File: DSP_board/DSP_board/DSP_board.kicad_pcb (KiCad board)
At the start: 4 copper layers, 134.2 x 94.8 mm, 94 parts, among them IC1 SN74S1053NSR, IC5 F280025CPNQR, J1 Conn_01x02, J2 Conn_01x02, J3 Conn_01x02, J4 Conn_01x02, J5 1-84981-0, J6 Conn_01x02, J7 Conn_02x10_Odd_Even, J8 Conn_02x06_Odd_Even, J9 Conn_02x06_Odd_Even

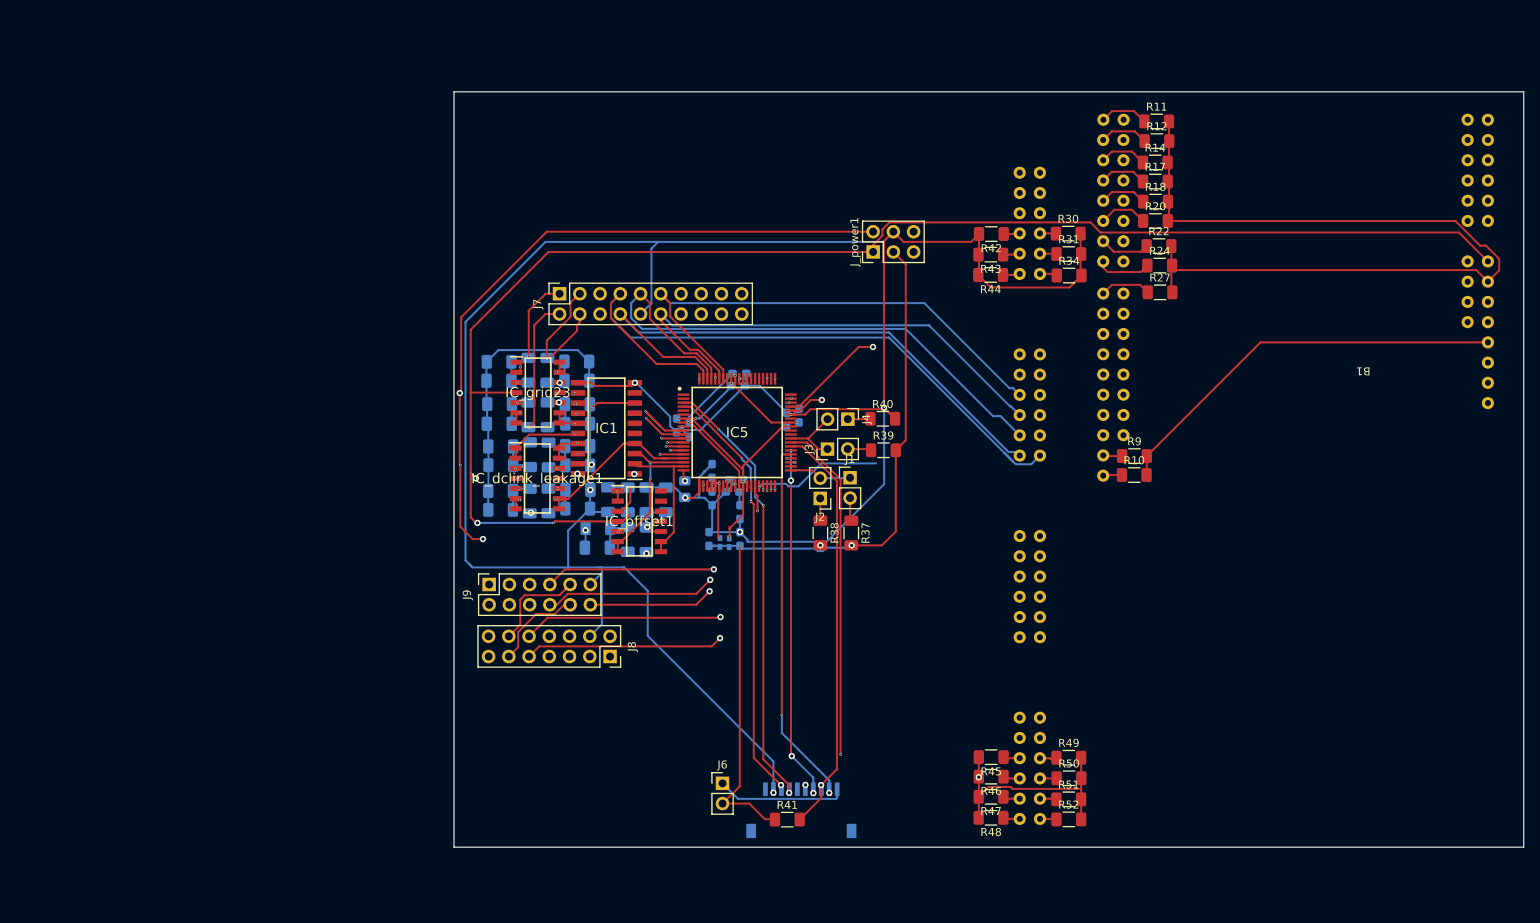
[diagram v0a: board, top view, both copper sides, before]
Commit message: header design
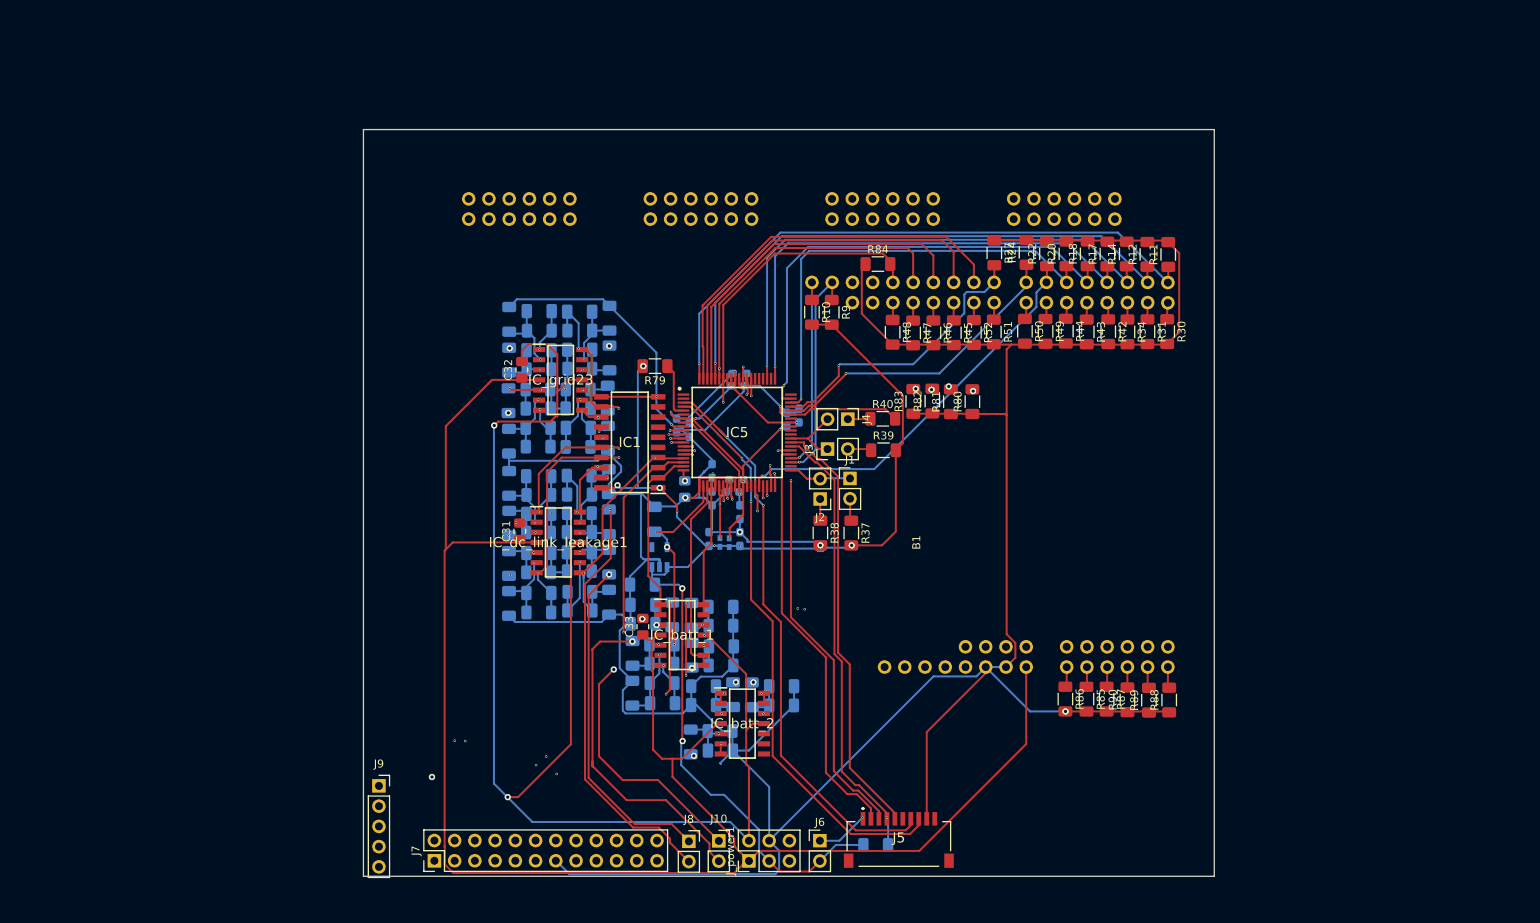
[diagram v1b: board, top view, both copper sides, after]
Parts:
- removed IC_dclink_leakage1, IC_offset1: LM324DR, lm324:SOIC127P600X175-14N
- added C12: CAP, Capacitor_SMD:C_1206_3216Metric_Pad1.33x1.80mm_HandSolder, B.Cu at (108.1, 74.1)
- added C13: CAP, Capacitor_SMD:C_1206_3216Metric_Pad1.33x1.80mm_HandSolder, B.Cu at (108.1, 109.5)
- added C20: CAP, Capacitor_SMD:C_1206_3216Metric_Pad1.33x1.80mm_HandSolder, B.Cu at (113.2, 111.7)
- added C21: CAP, Capacitor_SMD:C_1206_3216Metric_Pad1.33x1.80mm_HandSolder, B.Cu at (113.2, 74.2)
- added C22: CAP, Capacitor_SMD:C_1206_3216Metric_Pad1.33x1.80mm_HandSolder, B.Cu at (113.2, 97.2)
- added C23: CAP, Capacitor_SMD:C_1206_3216Metric_Pad1.33x1.80mm_HandSolder, B.Cu at (138.5, 121.2)
- added C24: CAP, Capacitor_SMD:C_1206_3216Metric_Pad1.33x1.80mm_HandSolder, B.Cu at (113.2, 104.4)
- added C25: CAP, Capacitor_SMD:C_1206_3216Metric_Pad1.33x1.80mm_HandSolder, B.Cu at (113.2, 101.9)
- added C26: CAP, Capacitor_SMD:C_1206_3216Metric_Pad1.33x1.80mm_HandSolder, B.Cu at (121.1, 111.0)
- added C27: CAP, Capacitor_SMD:C_1206_3216Metric_Pad1.33x1.80mm_HandSolder, B.Cu at (121.1, 108.5)
- added C28: CAP, Capacitor_SMD:C_1206_3216Metric_Pad1.33x1.80mm_HandSolder, B.Cu at (123.6, 123.3)
- added C29: CAP, Capacitor_SMD:C_1206_3216Metric_Pad1.33x1.80mm_HandSolder, B.Cu at (122.6, 100.3)
- added C30: CAP, Capacitor_SMD:C_1206_3216Metric_Pad1.33x1.80mm_HandSolder, B.Cu at (130.9, 111.2)
- added C31: CAP, Capacitor_SMD:C_0805_2012Metric_Pad1.18x1.45mm_HandSolder, F.Cu at (105.7, 101.8)
- added C32: CAP, Capacitor_SMD:C_0805_2012Metric_Pad1.18x1.45mm_HandSolder, F.Cu at (105.9, 81.5)
- added C33: CAP, Capacitor_SMD:C_0805_2012Metric_Pad1.18x1.45mm_HandSolder, F.Cu at (121.1, 113.7)
- added C5: CAP, Capacitor_SMD:C_1206_3216Metric_Pad1.33x1.80mm_HandSolder, B.Cu at (108.1, 104.5)
- added C6: CAP, Capacitor_SMD:C_1206_3216Metric_Pad1.33x1.80mm_HandSolder, B.Cu at (108.1, 99.6)
- added C8: CAP, Capacitor_SMD:C_1206_3216Metric_Pad1.33x1.80mm_HandSolder, B.Cu at (128.8, 123.6)
- added IC_batt_1: LM324DR, lm324:SOIC127P600X175-14N, F.Cu at (126.0, 114.8)
- added IC_batt_2: LM324DR, lm324:SOIC127P600X175-14N, F.Cu at (133.6, 125.9)
- added IC_dc_link_leakage1: LM324DR, lm324:SOIC127P600X175-14N, F.Cu at (110.5, 103.2)
- added J10: Conn_02x01, Connector_PinSocket_2.54mm:PinSocket_1x02_P2.54mm_Vertical, F.Cu at (130.7, 140.6)
- added LDO1: NCV8114ASN165T1G, ldo_ncv118:SOT95P275X110-5N, B.Cu at (123.2, 105.0)
- added R53: R, Resistor_SMD:R_1206_3216Metric_Pad1.30x1.75mm_HandSolder, B.Cu at (108.0, 91.1)
- added R54: R, Resistor_SMD:R_1206_3216Metric_Pad1.30x1.75mm_HandSolder, B.Cu at (108.1, 97.2)
- added R55: R, Resistor_SMD:R_1206_3216Metric_Pad1.30x1.75mm_HandSolder, B.Cu at (108.1, 111.9)
- added R56: R, Resistor_SMD:R_1206_3216Metric_Pad1.30x1.75mm_HandSolder, B.Cu at (132.4, 122.3)
- added R57: R, Resistor_SMD:R_1206_3216Metric_Pad1.30x1.75mm_HandSolder, B.Cu at (127.1, 128.2)
- added R58: R, Resistor_SMD:R_1206_3216Metric_Pad1.30x1.75mm_HandSolder, B.Cu at (134.8, 122.3)
- added R59: R, Resistor_SMD:R_1206_3216Metric_Pad1.30x1.75mm_HandSolder, B.Cu at (116.7, 90.1)
- added R60: R, Resistor_SMD:R_1206_3216Metric_Pad1.30x1.75mm_HandSolder, B.Cu at (113.2, 76.6)
- added R61: R, Resistor_SMD:R_1206_3216Metric_Pad1.30x1.75mm_HandSolder, B.Cu at (116.9, 110.7)
- added R62: R, Resistor_SMD:R_1206_3216Metric_Pad1.30x1.75mm_HandSolder, B.Cu at (113.0, 91.2)
- added R63: R, Resistor_SMD:R_1206_3216Metric_Pad1.30x1.75mm_HandSolder, B.Cu at (113.1, 94.8)
- added R64: R, Resistor_SMD:R_1206_3216Metric_Pad1.30x1.75mm_HandSolder, B.Cu at (113.2, 109.4)
- added R65: R, Resistor_SMD:R_1206_3216Metric_Pad1.30x1.75mm_HandSolder, B.Cu at (138.5, 123.6)
- added R66: R, Resistor_SMD:R_1206_3216Metric_Pad1.30x1.75mm_HandSolder, B.Cu at (116.9, 105.6)
- added R67: R, Resistor_SMD:R_1206_3216Metric_Pad1.30x1.75mm_HandSolder, B.Cu at (117.0, 75.0)
- added R68: R, Resistor_SMD:R_1206_3216Metric_Pad1.30x1.75mm_HandSolder, B.Cu at (113.0, 84.0)
- added R69: R, Resistor_SMD:R_1206_3216Metric_Pad1.30x1.75mm_HandSolder, B.Cu at (116.8, 95.5)
- added R70: R, Resistor_SMD:R_1206_3216Metric_Pad1.30x1.75mm_HandSolder, B.Cu at (113.2, 106.8)
- added R71: R, Resistor_SMD:R_1206_3216Metric_Pad1.30x1.75mm_HandSolder, B.Cu at (116.9, 100.6)
- added R72: R, Resistor_SMD:R_1206_3216Metric_Pad1.30x1.75mm_HandSolder, B.Cu at (113.2, 99.5)
- added R73: R, Resistor_SMD:R_1206_3216Metric_Pad1.30x1.75mm_HandSolder, B.Cu at (121.2, 113.4)
- added R74: R, Resistor_SMD:R_1206_3216Metric_Pad1.30x1.75mm_HandSolder, B.Cu at (123.5, 120.8)
- added R75: R, Resistor_SMD:R_1206_3216Metric_Pad1.30x1.75mm_HandSolder, B.Cu at (124.8, 112.3)
- added R76: R, Resistor_SMD:R_1206_3216Metric_Pad1.30x1.75mm_HandSolder, B.Cu at (130.9, 113.6)
- added R77: R, Resistor_SMD:R_1206_3216Metric_Pad1.30x1.75mm_HandSolder, B.Cu at (127.2, 112.3)
- added R78: R, Resistor_SMD:R_1206_3216Metric_Pad1.30x1.75mm_HandSolder, B.Cu at (119.8, 122.1)
- added R79: R, Resistor_SMD:R_1206_3216Metric_Pad1.30x1.75mm_HandSolder, F.Cu at (122.7, 81.0)
- added R80: R, Resistor_SMD:R_1206_3216Metric_Pad1.30x1.75mm_HandSolder, F.Cu at (162.5, 85.5)
- added R81: R, Resistor_SMD:R_1206_3216Metric_Pad1.30x1.75mm_HandSolder, F.Cu at (159.8, 85.5)
- added R82: R, Resistor_SMD:R_1206_3216Metric_Pad1.30x1.75mm_HandSolder, F.Cu at (157.5, 85.4)
- added R83: R, Resistor_SMD:R_1206_3216Metric_Pad1.30x1.75mm_HandSolder, F.Cu at (155.1, 85.5)
- added R84: R, Resistor_SMD:R_1206_3216Metric_Pad1.30x1.75mm_HandSolder, F.Cu at (150.6, 68.2)
- added R85: R, Resistor_SMD:R_1206_3216Metric_Pad1.30x1.75mm_HandSolder, F.Cu at (176.8, 122.8)
- added R86: R, Resistor_SMD:R_1206_3216Metric_Pad1.30x1.75mm_HandSolder, F.Cu at (174.2, 122.8)
- added R87: R, Resistor_SMD:R_1206_3216Metric_Pad1.30x1.75mm_HandSolder, F.Cu at (179.3, 122.8)
- added R88: R, Resistor_SMD:R_1206_3216Metric_Pad1.30x1.75mm_HandSolder, F.Cu at (187.2, 122.9)
- added R89: R, Resistor_SMD:R_1206_3216Metric_Pad1.30x1.75mm_HandSolder, F.Cu at (184.7, 123.0)
- added R90: R, Resistor_SMD:R_1206_3216Metric_Pad1.30x1.75mm_HandSolder, F.Cu at (181.9, 122.9)
- J5: moved to F.Cu
- J7: value Conn_02x10_Odd_Even -> Conn_02x12_Odd_Even; footprint Connector_PinSocket_2.54mm:PinSocket_2x10_P2.54mm_Vertical -> Connector_PinHeader_2.54mm:PinHeader_2x12_P2.54mm_Vertical
- J8: value Conn_02x06_Odd_Even -> Conn_02x01; footprint Connector_PinSocket_2.54mm:PinSocket_2x07_P2.54mm_Vertical -> Connector_PinSocket_2.54mm:PinSocket_1x02_P2.54mm_Vertical
- J9: value Conn_02x06_Odd_Even -> Conn_01x05; footprint Connector_PinSocket_2.54mm:PinSocket_2x06_P2.54mm_Vertical -> Connector_PinSocket_2.54mm:PinSocket_1x05_P2.54mm_Vertical
- R41: moved to B.Cu
- moved J_power1 78.0 mm to (134.4, 143.1)
- moved J7 72.9 mm to (95.0, 143.1)
- moved B1 67.0 mm to (155.0, 108.3), turned to 90 degrees
- moved R52 62.3 mm to (162.7, 76.8), turned to -90 degrees
- moved R48 62.2 mm to (152.5, 76.8), turned to -90 degrees
- moved R51 59.4 mm to (165.2, 76.7), turned to -90 degrees
- moved R47 59.0 mm to (155.1, 76.9), turned to -90 degrees
- moved R50 56.4 mm to (169.1, 76.7), turned to -90 degrees
- moved R46 56.2 mm to (157.6, 76.8), turned to -90 degrees
- moved R49 53.6 mm to (171.7, 76.7), turned to -90 degrees
- moved R45 53.5 mm to (160.2, 76.8), turned to -90 degrees
- moved C10 47.1 mm to (130.9, 129.3), turned to 0 degrees
- moved R10 45.3 mm to (142.3, 74.3), turned to -90 degrees
- moved R9 42.1 mm to (144.8, 74.3), turned to -90 degrees
- moved R33 36.0 mm to (130.8, 126.8), turned to 180 degrees
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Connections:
- B1 pad 102: VSI11 -> unconnected-(B1-Pad102)
- B1 pad 103: VSI21 -> unconnected-(B1-Pad103)
- B1 pad 104: VSI31 -> unconnected-(B1-Pad104)
- B1 pad 14: unconnected-(B1-Pad14) -> OCD_grid1
- B1 pad 15: unconnected-(B1-Pad15) -> OCD_grd2
- B1 pad 16: unconnected-(B1-Pad16) -> OCD_grid3
- B1 pad 17: unconnected-(B1-Pad17) -> relay_3
- B1 pad 18: unconnected-(B1-Pad18) -> relay_2
- B1 pad 19: unconnected-(B1-Pad19) -> relay_1
- B1 pad 26: unconnected-(B1-Pad26) -> batt_ready
- B1 pad 27: unconnected-(B1-Pad27) -> batt_fault
- B1 pad 28: unconnected-(B1-Pad28) -> DAB2_PWM22
- B1 pad 29: unconnected-(B1-Pad29) -> DAB2_PWM21
- B1 pad 30: unconnected-(B1-Pad30) -> DAB2_PWM12
- B1 pad 31: unconnected-(B1-Pad31) -> DAB2_PWM11
- B1 pad 32: unconnected-(B1-Pad32) -> DAB1PWM22
- B1 pad 33: unconnected-(B1-Pad33) -> DAB1PWM21
- B1 pad 34: unconnected-(B1-Pad34) -> DAB1PWM12
- B1 pad 35: unconnected-(B1-Pad35) -> DAB1PWM11
- B1 pad 36: unconnected-(B1-Pad36) -> VSI32
- B1 pad 37: unconnected-(B1-Pad37) -> VSI31
- B1 pad 38: unconnected-(B1-Pad38) -> VSI22
- B1 pad 39: unconnected-(B1-Pad39) -> VSI21
- B1 pad 40: unconnected-(B1-Pad40) -> VSI12
- B1 pad 41: unconnected-(B1-Pad41) -> VSI11
- B1 pad 46: unconnected-(B1-Pad46) -> vsi_ready
- B1 pad 47: unconnected-(B1-Pad47) -> vsi_fault
- B1 pad 48: unconnected-(B1-Pad48) -> OCD_leakage
- B1 pad 49: unconnected-(B1-Pad49) -> dc_fault
- B1 pad 50: unconnected-(B1-Pad50) -> dc_ready
- B1 pad 60: DAB1PWM22 -> unconnected-(B1-Pad60)
- B1 pad 61: DAB1PWM21 -> unconnected-(B1-Pad61)
- B1 pad 62: DAB1PWM12 -> unconnected-(B1-Pad62)
- B1 pad 63: DAB1PWM11 -> unconnected-(B1-Pad63)
- B1 pad 66: DAB2_PWM22 -> unconnected-(B1-Pad66)
- B1 pad 67: DAB2_PWM21 -> unconnected-(B1-Pad67)
- B1 pad 68: DAB2_PWM12 -> unconnected-(B1-Pad68)
- B1 pad 69: DAB2_PWM11 -> unconnected-(B1-Pad69)
- B1 pad 84: OCD_grid1 -> unconnected-(B1-Pad84)
- B1 pad 90: OCD_grd2 -> unconnected-(B1-Pad90)
- B1 pad 91: OCD_grid3 -> unconnected-(B1-Pad91)
- B1 pad 92: vsi_fault -> unconnected-(B1-Pad92)
- B1 pad 93: vsi_ready -> unconnected-(B1-Pad93)
- B1 pad 96: VSI12 -> unconnected-(B1-Pad96)
- B1 pad 97: VSI22 -> unconnected-(B1-Pad97)
- B1 pad 98: VSI32 -> unconnected-(B1-Pad98)
- C10 pad 2: offset_v -> ctrl_gnd
- C11 pad 1: Net-(C11-Pad1) -> Vgrid3_sense
- C11 pad 2: offset_v -> Net-(C11-Pad2)
- C14 pad 1: Net-(C14-Pad1) -> Igrid1_sense
- C14 pad 2: ctrl_gnd -> Net-(C14-Pad2)
- C15 pad 2: offset_v -> Vgrid2_sense
- IC1 pad 13: Igrid3_sense -> Vgrid2_sense
- IC1 pad 14: Vgrid3_sense -> Igrid3_sense
- IC1 pad 15: Vgrid2_sense -> Vgrid3_sense
- IC1 pad 17: I_leackage -> Vgrid1_sense
- IC1 pad 18: Vgrid1_sense -> I_leackage
- IC1 pad 19: unconnected-(IC1-Pad19) -> offset_v
- IC1 pad 8: offset_v -> unconnected-(IC1-Pad8)
- IC5 pad 11: Igrid3_sense -> Vgrid2_sense
- IC5 pad 12: Vgrid3_sense -> Igrid3_sense
- IC5 pad 13: Vgrid2_sense -> Vgrid3_sense
- IC5 pad 15: I_leackage -> Vgrid1_sense
- IC5 pad 16: Vgrid1_sense -> I_leackage
- IC5 pad 23: unconnected-(IC5-Pad23) -> ADC1
- IC5 pad 24: unconnected-(IC5-Pad24) -> ADC2
- IC5 pad 27: unconnected-(IC5-Pad27) -> ADC3
- IC5 pad 28: unconnected-(IC5-Pad28) -> ADC4
- IC5 pad 29: unconnected-(IC5-Pad29) -> ADC5
- IC5 pad 35: dc_ready -> OCD_grid1
- IC5 pad 37: dc_fault -> OCD_grd2
- IC5 pad 38: OCD_leakage -> OCD_grid3
- IC5 pad 5: unconnected-(IC5-Pad5) -> Net-(IC5-Pad5)
- IC5 pad 56: /controller_sheet/en_dab -> /controller_sheet/en_vsi
- IC5 pad 57: /controller_sheet/en_vsi -> /controller_sheet/en_dab
- IC5 pad 67: unconnected-(IC5-Pad67) -> relay_3
- IC5 pad 68: unconnected-(IC5-Pad68) -> relay_2
- IC5 pad 69: unconnected-(IC5-Pad69) -> relay_1
- IC5 pad 77: OCD_grid3 -> OCD_leakage
- IC5 pad 78: OCD_grd2 -> dc_fault
- IC5 pad 79: OCD_grid1 -> dc_ready
- IC_grid23 pad 13: Igrid2_sense -> Net-(C21-Pad2)
- IC_grid23 pad 2: Igrid3_sense -> Net-(C12-Pad2)
- IC_grid23 pad 6: Vgrid3_sense -> Net-(C11-Pad2)
- IC_grid23 pad 9: Vgrid2_sense -> Net-(C15-Pad1)
- J5 pad 3: TMS -> TDO
- J5 pad 4: TDO -> TMS
- J7 pad 1: Igrid3 -> relay_3
- J7 pad 10: ctrl_gnd -> Igrid1
- J7 pad 11: vsi_ready -> OCD_grd2
- J7 pad 12: vsi_fault -> OCD_grid1
- J7 pad 13: VSI31 -> ctrl_gnd
- J7 pad 14: VSI32 -> OCD_grid3
- J7 pad 15: VSI21 -> vsi_fault
- J7 pad 16: VSI22 -> vsi_ready
- J7 pad 17: VSI11 -> VSI31
- J7 pad 18: VSI12 -> VSI32
- J7 pad 19: SCL -> VSI21
- J7 pad 2: Vgrid3 -> unconnected-(J7-Pad2)
- J7 pad 20: SDA -> VSI22
- J7 pad 3: Igrid2 -> relay_2
- J7 pad 4: Vgrid2 -> relay_1
- J7 pad 5: Igrid1 -> Vgrid3
- J7 pad 6: Vgrid1 -> Igrid3
- J7 pad 7: OCD_grid1 -> Vgrid2
- J7 pad 8: OCD_grd2 -> Igrid2
- J7 pad 9: OCD_grid3 -> Vgrid1
- J8 pad 1: batt_curr_0 -> V_dc_link
- J8 pad 2: batt_v -> curr_leakeage_i
- J9 pad 1: curr_leakeage_i -> Analog_in1
- J9 pad 2: V_dc_link -> Analog_in2
- J9 pad 3: DAB1PWM21 -> Analog_in3
- J9 pad 4: DAB1PWM22 -> Analog_in4
- J9 pad 5: DAB1PWM11 -> Analog_in5
- R10 pad 2: FPGA_3v3 -> ctrl_3v3
- R13 pad 1: Net-(IC_offset1-Pad3) -> offset_v
- R13 pad 2: ctrl_15 -> Net-(C5-Pad1)
- R15 pad 1: Net-(IC_offset1-Pad3) -> offset_v
- R15 pad 2: ctrl_gnd -> Net-(C6-Pad1)
- R19 pad 1: offset_v -> Net-(C6-Pad1)
- R19 pad 2: Net-(C7-Pad1) -> Igrid1
- R25 pad 1: offset_v -> Vgrid1
- R25 pad 2: Net-(C10-Pad1) -> Net-(C5-Pad1)
- R26 pad 1: Net-(C10-Pad1) -> ctrl_gnd
- R26 pad 2: Igrid1 -> Net-(C12-Pad2)
- R27 pad 1: /controller_sheet/en_dab -> ctrl_gnd
- R27 pad 2: ctrl_gnd -> /controller_sheet/en_dab
- R28 pad 1: offset_v -> ctrl_gnd
- R28 pad 2: Net-(C11-Pad1) -> Net-(C14-Pad2)
- R29 pad 1: Vgrid1 -> ctrl_gnd
- R29 pad 2: Net-(C11-Pad1) -> Net-(C11-Pad2)
- R30 pad 1: VSI32 -> VSI11
- R31 pad 1: VSI22 -> VSI12
- R32 pad 2: Net-(C14-Pad1) -> Net-(C8-Pad1)
- R33 pad 1: V_dc_link -> ctrl_gnd
- R33 pad 2: Net-(C14-Pad1) -> Net-(C10-Pad1)
- R34 pad 1: VSI12 -> VSI21
- R35 pad 1: Net-(C15-Pad1) -> ctrl_gnd
- R35 pad 2: curr_leakeage_i -> Net-(C13-Pad2)
- R36 pad 1: offset_v -> Net-(C12-Pad2)
- R36 pad 2: Net-(C15-Pad1) -> Igrid3_sense
- R42 pad 1: VSI31 -> VSI22
- R43 pad 1: VSI21 -> VSI31
- R44 pad 1: VSI11 -> VSI32
- R9 pad 2: FPGA_3v3 -> ctrl_3v3
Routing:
- net relay_1: track 0.00 -> 149.2 mm, vias 0 -> 2
- net relay_3: track 0.00 -> 146.3 mm, vias 0 -> 2
- net relay_2: track 0.00 -> 144.4 mm, vias 0 -> 2
- net DAB1PWM22: track 87.3 -> 2.20 mm
- net DAB1PWM21: track 86.7 -> 2.14 mm
- net DAB1PWM11: track 79.5 -> 2.11 mm
- net DAB1PWM12: track 78.5 -> 2.12 mm
- net ctrl_gnd: track 609.5 -> 534.1 mm, vias 12 -> 9
- net DAB2_PWM22: track 70.4 -> 2.18 mm
- net DAB2_PWM11: track 68.7 -> 2.24 mm
- net DAB2_PWM21: track 68.6 -> 2.25 mm
- net VSI11: track 40.6 -> 104.5 mm
- net DAB2_PWM12: track 66.0 -> 2.24 mm
- net vsi_fault: track 62.1 -> 125.3 mm, vias 0 -> 2
- net Igrid2: track 9.86 -> 70.6 mm
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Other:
- board size 134.2 x 94.8 mm -> 106.8 x 93.7 mm

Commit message: review changes
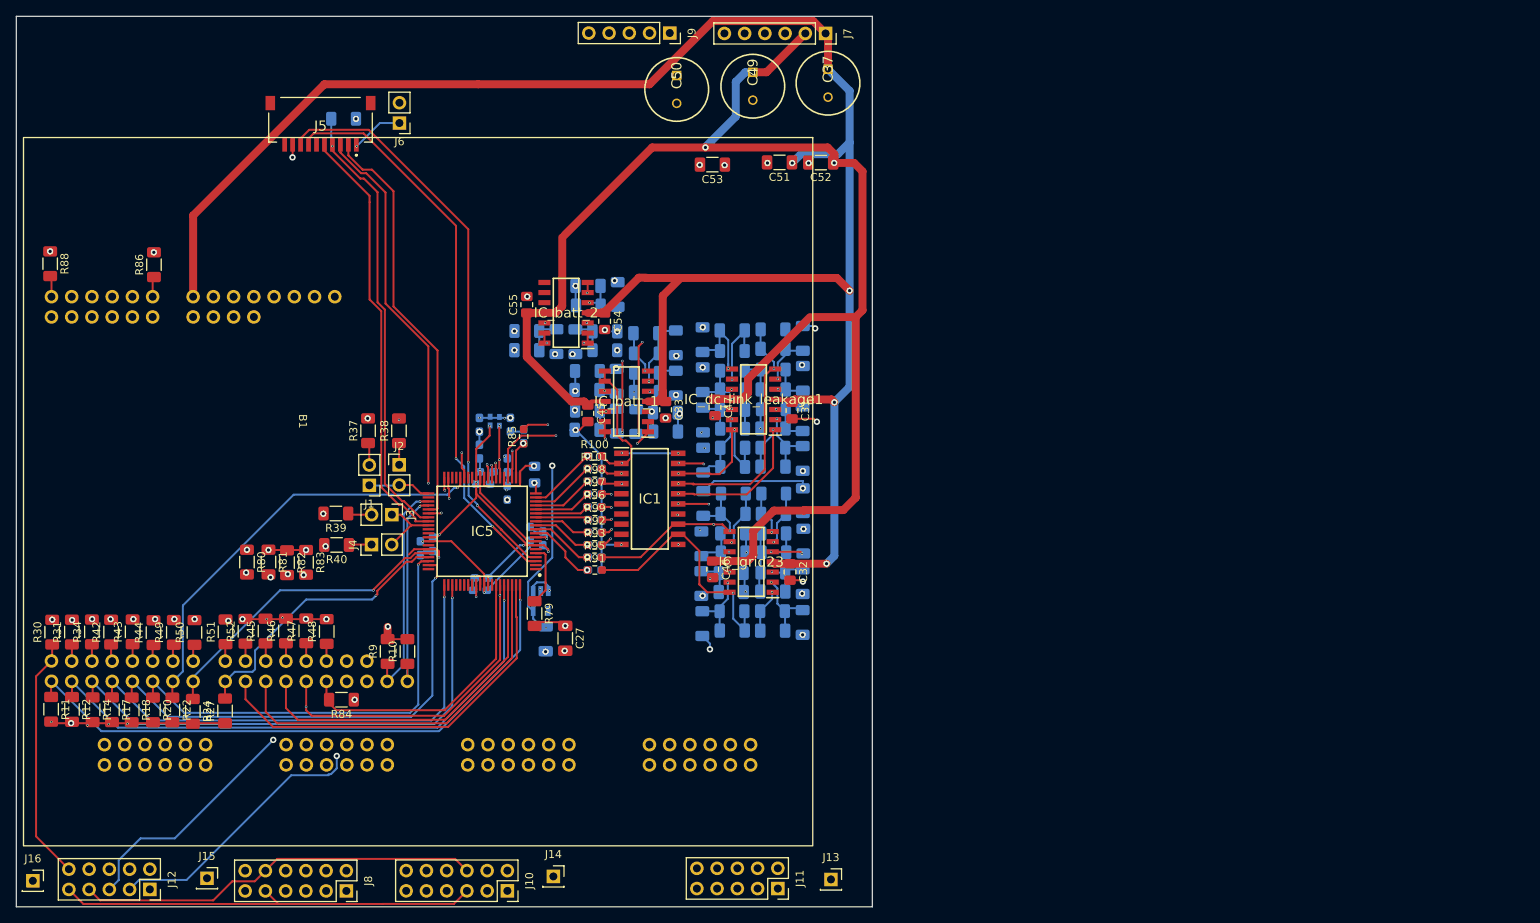
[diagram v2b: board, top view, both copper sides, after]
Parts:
- removed J_power1: Conn_02x03_Counter_Clockwise, Connector_PinHeader_2.54mm:PinHeader_2x03_P2.54mm_Vertical
- removed R87, R89, R90: R, Resistor_SMD:R_1206_3216Metric_Pad1.30x1.75mm_HandSolder
- added C34: CAP, Capacitor_SMD:C_0603_1608Metric_Pad1.08x0.95mm_HandSolder, B.Cu at (115.1, 106.6)
- added C35: CAP, Capacitor_SMD:C_0603_1608Metric_Pad1.08x0.95mm_HandSolder, B.Cu at (115.1, 101.9)
- added C36: CAP, Capacitor_SMD:C_0603_1608Metric_Pad1.08x0.95mm_HandSolder, B.Cu at (115.1, 103.4)
- added C37: ESK107M050AG3EA, electrolytic_cap:CAPPRD350W60D800H1250, F.Cu at (144.4, 43.8)
- added C38: CAP, Capacitor_SMD:C_0603_1608Metric_Pad1.08x0.95mm_HandSolder, B.Cu at (115.1, 105.0)
- added C39: CAP, Capacitor_SMD:C_0603_1608Metric_Pad1.08x0.95mm_HandSolder, B.Cu at (115.0, 98.7)
- added C40: CAP, Capacitor_SMD:C_0603_1608Metric_Pad1.08x0.95mm_HandSolder, B.Cu at (115.1, 97.1)
- added C41: CAP, Capacitor_SMD:C_0603_1608Metric_Pad1.08x0.95mm_HandSolder, B.Cu at (115.1, 95.5)
- added C42: CAP, Capacitor_SMD:C_0603_1608Metric_Pad1.08x0.95mm_HandSolder, B.Cu at (115.1, 100.3)
- added C43: CAP, Capacitor_SMD:C_0603_1608Metric_Pad1.08x0.95mm_HandSolder, B.Cu at (115.1, 92.3)
- added C44: CAP, Capacitor_SMD:C_0603_1608Metric_Pad1.08x0.95mm_HandSolder, B.Cu at (115.1, 93.9)
- added C45: CAP, Capacitor_SMD:C_0805_2012Metric_Pad1.18x1.45mm_HandSolder, F.Cu at (114.2, 87.0)
- added C46: CAP, Capacitor_SMD:C_0805_2012Metric_Pad1.18x1.45mm_HandSolder, F.Cu at (129.9, 106.5)
- added C47: CAP, Capacitor_SMD:C_0805_2012Metric_Pad1.18x1.45mm_HandSolder, F.Cu at (130.2, 86.2)
- added C48: CAP, Capacitor_SMD:C_0603_1608Metric_Pad1.08x0.95mm_HandSolder, B.Cu at (106.2, 89.8)
- added C49: ESK107M050AG3EA, electrolytic_cap:CAPPRD350W60D800H1250, F.Cu at (134.9, 44.1)
- added C50: ESK107M050AG3EA, electrolytic_cap:CAPPRD350W60D800H1250, F.Cu at (125.4, 44.5)
- added C51: CAP, Capacitor_SMD:C_1206_3216Metric_Pad1.33x1.80mm_HandSolder, F.Cu at (138.3, 55.5)
- added C52: CAP, Capacitor_SMD:C_1206_3216Metric_Pad1.33x1.80mm_HandSolder, F.Cu at (143.5, 55.5)
- added C53: CAP, Capacitor_SMD:C_1206_3216Metric_Pad1.33x1.80mm_HandSolder, F.Cu at (129.9, 55.7)
- added C54: CAP, Capacitor_SMD:C_0805_2012Metric_Pad1.18x1.45mm_HandSolder, F.Cu at (116.3, 75.4)
- added C55: CAP, Capacitor_SMD:C_0805_2012Metric_Pad1.18x1.45mm_HandSolder, F.Cu at (106.6, 73.3)
- added J11: Conn_02x05_Odd_Even, Connector_PinSocket_2.54mm:PinSocket_2x05_P2.54mm_Vertical, F.Cu at (138.1, 146.6)
- added J12: Conn_02x05_Odd_Even, Connector_PinSocket_2.54mm:PinSocket_2x05_P2.54mm_Vertical, F.Cu at (59.2, 146.7)
- added J13: Conn_01x01_Female, Connector_PinSocket_2.54mm:PinSocket_1x01_P2.54mm_Vertical, F.Cu at (144.7, 145.5)
- added J14: Conn_01x01_Female, Connector_PinSocket_2.54mm:PinSocket_1x01_P2.54mm_Vertical, F.Cu at (109.9, 145.1)
- added J15: Conn_01x01_Female, Connector_PinSocket_2.54mm:PinSocket_1x01_P2.54mm_Vertical, F.Cu at (66.4, 145.3)
- added J16: Conn_01x01_Female, Connector_PinSocket_2.54mm:PinSocket_1x01_P2.54mm_Vertical, F.Cu at (44.6, 145.6)
- added R100: R, Resistor_SMD:R_0603_1608Metric_Pad0.98x0.95mm_HandSolder, F.Cu at (115.1, 92.3)
- added R101: R, Resistor_SMD:R_0603_1608Metric_Pad0.98x0.95mm_HandSolder, F.Cu at (115.1, 93.9)
- added R91: R, Resistor_SMD:R_0603_1608Metric_Pad0.98x0.95mm_HandSolder, F.Cu at (115.1, 106.6)
- added R92: R, Resistor_SMD:R_0603_1608Metric_Pad0.98x0.95mm_HandSolder, F.Cu at (115.1, 101.9)
- added R93: R, Resistor_SMD:R_0603_1608Metric_Pad0.98x0.95mm_HandSolder, F.Cu at (115.1, 103.5)
- added R95: R, Resistor_SMD:R_0603_1608Metric_Pad0.98x0.95mm_HandSolder, F.Cu at (115.1, 105.0)
- added R96: R, Resistor_SMD:R_0603_1608Metric_Pad0.98x0.95mm_HandSolder, F.Cu at (115.0, 98.7)
- added R97: R, Resistor_SMD:R_0603_1608Metric_Pad0.98x0.95mm_HandSolder, F.Cu at (115.1, 97.1)
- added R98: R, Resistor_SMD:R_0603_1608Metric_Pad0.98x0.95mm_HandSolder, F.Cu at (115.1, 95.5)
- added R99: R, Resistor_SMD:R_0603_1608Metric_Pad0.98x0.95mm_HandSolder, F.Cu at (115.1, 100.3)
- C27: moved to F.Cu
- J10, J8: value Conn_02x01 -> Conn_02x06_Odd_Even; footprint Connector_PinSocket_2.54mm:PinSocket_1x02_P2.54mm_Vertical -> Connector_PinSocket_2.54mm:PinSocket_2x06_P2.54mm_Vertical
- J7: value Conn_02x12_Odd_Even -> Conn_01x06; footprint Connector_PinHeader_2.54mm:PinHeader_2x12_P2.54mm_Vertical -> Connector_PinSocket_2.54mm:PinSocket_1x06_P2.54mm_Vertical
- R85: footprint Resistor_SMD:R_1206_3216Metric_Pad1.30x1.75mm_HandSolder -> Resistor_SMD:R_0603_1608Metric_Pad0.98x0.95mm_HandSolder
- moved R11 151.4 mm to (46.9, 124.1), turned to -90 degrees
- moved R88 150.7 mm to (46.7, 68.2), turned to -90 degrees
- moved R12 146.6 mm to (49.5, 124.1), turned to -90 degrees
- moved R30 144.9 mm to (47.0, 114.4), turned to 90 degrees
- moved R14 141.8 mm to (52.1, 124.2), turned to -90 degrees
- moved R31 140.2 mm to (49.5, 114.4), turned to 90 degrees
- moved R17 137.4 mm to (54.5, 124.2), turned to -90 degrees
- moved R34 135.3 mm to (52.0, 114.4), turned to 90 degrees
- moved R18 132.9 mm to (57.0, 124.2), turned to -90 degrees
- moved R42 130.7 mm to (54.4, 114.4), turned to 90 degrees
- moved R20 128.1 mm to (59.6, 124.2), turned to -90 degrees
- moved R86 126.7 mm to (59.8, 68.3), turned to 90 degrees
- moved R43 125.5 mm to (57.1, 114.4), turned to 90 degrees
- moved R22 123.8 mm to (62.1, 124.2), turned to -90 degrees
- moved R44 120.6 mm to (59.7, 114.5), turned to 90 degrees
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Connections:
- B1 pad 15: OCD_grd2 -> unconnected-(B1-Pad15)
- B1 pad 16: OCD_grid3 -> unconnected-(B1-Pad16)
- B1 pad 17: relay_3 -> unconnected-(B1-Pad17)
- B1 pad 18: relay_2 -> unconnected-(B1-Pad18)
- C31 pad 2: ctrl_-15 -> ctrl_gnd
- C32 pad 2: ctrl_-15 -> ctrl_gnd
- C33 pad 2: ctrl_-15 -> ctrl_gnd
- IC5 pad 10: Igrid2_sense -> Igrid2_sense_f
- IC5 pad 11: Vgrid2_sense -> Vgrid2_sense_f
- IC5 pad 12: Igrid3_sense -> Igrid3_sense_f
- IC5 pad 13: Vgrid3_sense -> Vgrid3_sense_f
- IC5 pad 14: Igrid1_sense -> Igrid1_sense_f
- IC5 pad 15: Vgrid1_sense -> Vgrid1_sense_f
- IC5 pad 16: I_leackage -> I_leackage_f
- IC5 pad 17: Vdc_link -> Vdc_link_f
- IC5 pad 18: batt_curr_sense -> batt_curr_sense_f
- IC5 pad 19: batt_V_sense -> batt_V_sense_f
- IC5 pad 22: offset_v -> offset_f
- IC5 pad 37: OCD_grd2 -> unconnected-(IC5-Pad37)
- IC5 pad 38: OCD_grid3 -> unconnected-(IC5-Pad38)
- IC5 pad 67: relay_3 -> unconnected-(IC5-Pad67)
- IC5 pad 68: relay_2 -> unconnected-(IC5-Pad68)
- IC_batt_1 pad 1: batt_V_sense -> ADC1
- IC_batt_1 pad 2: batt_V_sense -> ADC1
- IC_batt_1 pad 8: ADC1 -> batt_V_sense
- IC_batt_1 pad 9: ADC1 -> batt_V_sense
- J10 pad 1: batt_v -> batt_curr_0
- J10 pad 2: batt_curr_0 -> batt_v
- J7 pad 1: relay_3 -> ctrl_15
- J7 pad 2: unconnected-(J7-Pad2) -> ctrl_-15
- J7 pad 3: relay_2 -> ctrl_3v3
- J7 pad 4: relay_1 -> ctrl_gnd
- J7 pad 5: Vgrid3 -> V_12
- J7 pad 6: Igrid3 -> 24_gnd
- J8 pad 1: V_dc_link -> curr_leakeage_i
- J8 pad 2: curr_leakeage_i -> V_dc_link
- R85 pad 1: OCD_grd2 -> offset_f
- R85 pad 2: ctrl_gnd -> offset_v
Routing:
- net ctrl_gnd: track 534.1 -> 126.9 mm, vias 9 -> 69
- net relay_3: track 146.3 -> 0.00 mm, vias 2 -> 0
- net relay_2: track 144.4 -> 0.00 mm, vias 2 -> 0
- net ctrl_3v3: track 159.2 -> 24.5 mm, vias 9 -> 12
- net OCD_grid3: track 115.6 -> 0.00 mm, vias 2 -> 0
- net OCD_grd2: track 115.0 -> 0.00 mm, vias 2 -> 0
- net VSI11: track 104.5 -> 30.7 mm
- net VSI21: track 101.6 -> 30.1 mm
- net VSI31: track 100.5 -> 30.1 mm
- net VSI12: track 99.8 -> 30.2 mm
- net VSI22: track 97.6 -> 31.0 mm
- net VSI32: track 96.4 -> 33.1 mm
- net V_dc_link: track 42.9 -> 102.8 mm
- net batt_fault: track 31.8 -> 82.0 mm
- net curr_leakeage_i: track 53.6 -> 95.6 mm
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- added copper zone on In1.Cu, net ctrl_3v3
- added copper zone on In2.Cu, net ctrl_gnd
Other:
- board size 106.8 x 93.7 mm -> 107.4 x 111.8 mm
